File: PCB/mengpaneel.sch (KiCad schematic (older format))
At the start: 296 parts, among them IC1 MAX7219CNG+, IC10 STM32F411CEU7, IC11 AD5204BRUZ10-REEL7, IC12 LTC3631EMS8E#TRPBF, IC13 LMV321AUIDBVR, IC2 MAX7219CNG+, IC3 MTCH6301-I_ML, IC4 LTC3121EDE#PBF, IC5 AD5204BRUZ10-REEL7, IC6 AD5204BRUZ10-REEL7, IC7 LM3480IM3-3.3_NOPB, IC8 AD5204BRUZ10-REEL7, IC9 AD5204BRUZ10-REEL7, J1 UJ2-MIBH-G-SMT-TR, J2 Screw_Terminal_01x03, J3 Screw_Terminal_01x14, J4 SJ-63053A, J5 SJ-63053A, J6 SJ-63053A, J7 SJ-63053A, SW1 SW_Push, SW2 SW_DPDT_x2, SW3 SW_DPST_x2, SW4 SW_DPST_x2, U11 Touchpad_mp, U13 Touchpad_mp_LR, U14 Touchpad_mp, U15 Touchpad_mp, U16 Touchpad_mp, U17 Touchpad_mp, U2 Touchpad_mp, U3 Touchpad_mp, U4 Touchpad_mp, U5 LM324N, U6 Touchpad_mp, U7 LM324N, U8 Touchpad_mp, Y1 8MHz

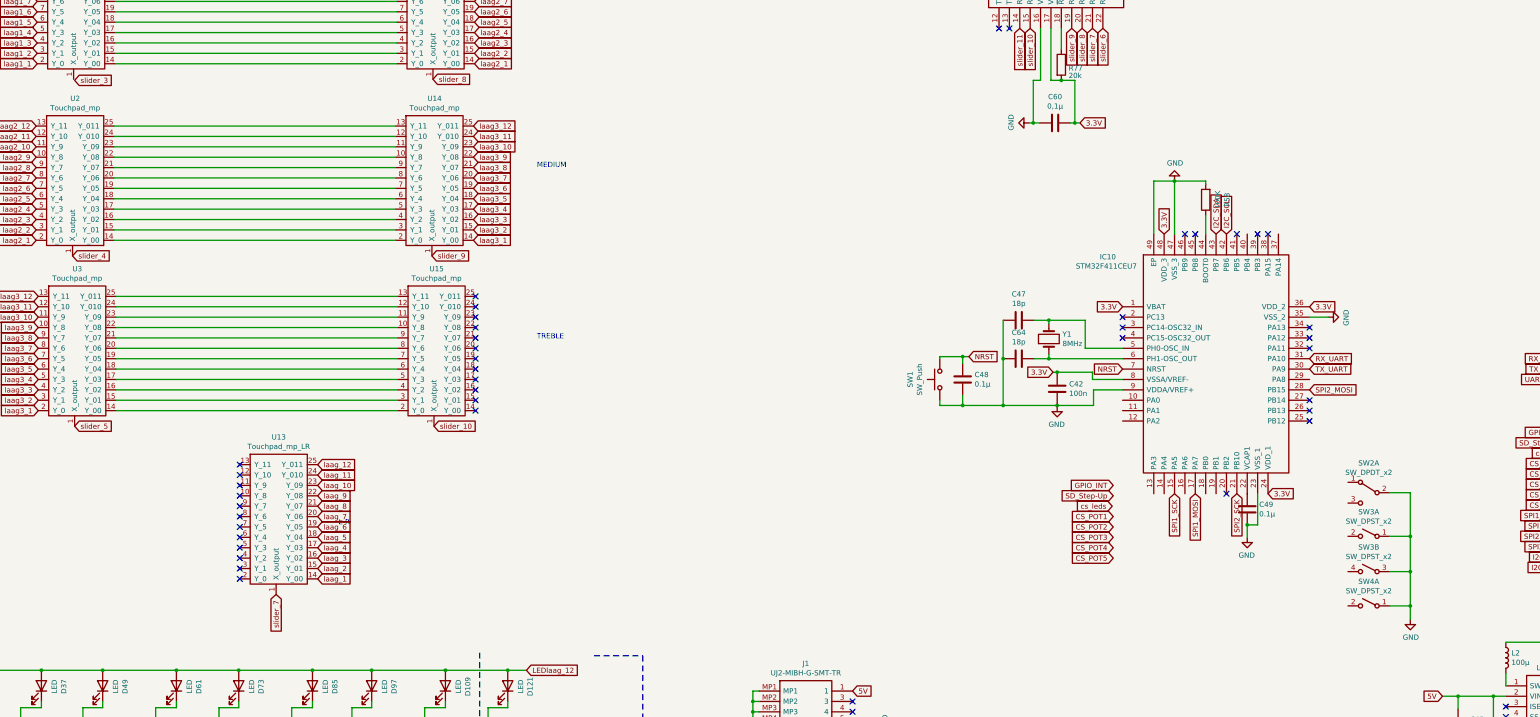
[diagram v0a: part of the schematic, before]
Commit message: PCB af nu wachten op de docenten hun feedback.
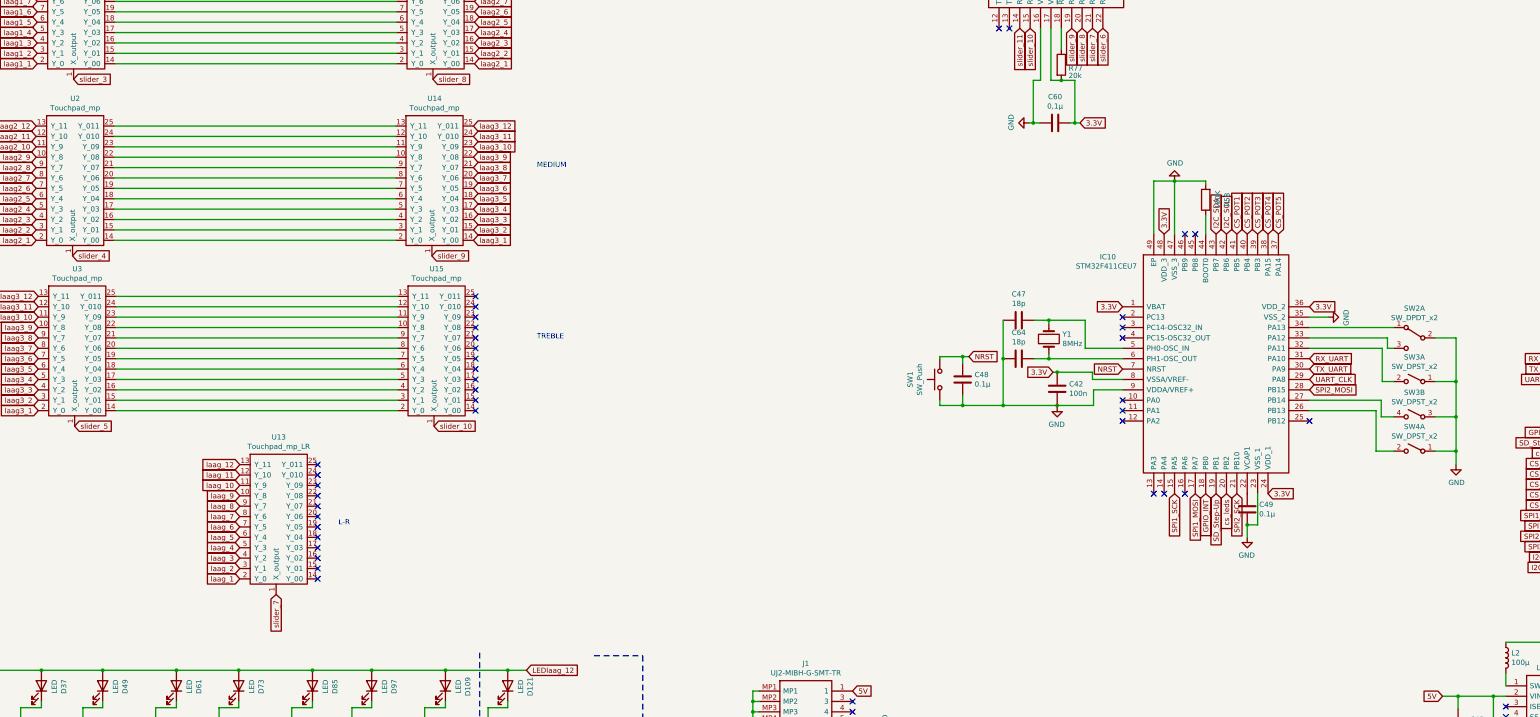
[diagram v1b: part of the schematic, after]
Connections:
- net CS_POT1: now also IC10.41 (PB5)
- net CS_POT2: now also IC10.40 (PB4)
- net CS_POT3: now also IC10.39 (PB3)
- net CS_POT4: now also IC10.38 (PA15)
- net CS_POT5: now also IC10.37 (PA14)
- net GPIO_INT: now also IC10.18 (PB0)
- net SD_Step-Up: now also IC10.19 (PB1)
- net UART_CLK: now also IC10.29 (PA8)
- net cs_leds: now also IC10.20 (PB2)
- net laag_1: now also U13.2 (Y_0); no longer U13.14 (Y_00)
- net laag_10: now also U13.11 (Y_9); no longer U13.23 (Y_09)
- net laag_11: now also U13.12 (Y_10); no longer U13.24 (Y_010)
- net laag_12: now also U13.13 (Y_11); no longer U13.25 (Y_011)
- net laag_2: now also U13.3 (Y_1); no longer U13.15 (Y_01)
- net laag_3: now also U13.4 (Y_2); no longer U13.16 (Y_02)
- net laag_4: now also U13.5 (Y_3); no longer U13.17 (Y_03)
- net laag_5: now also U13.6 (Y_4); no longer U13.18 (Y_04)
- net laag_6: now also U13.7 (Y_5); no longer U13.19 (Y_05)
- net laag_7: now also U13.8 (Y_6); no longer U13.20 (Y_06)
- net laag_8: now also U13.9 (Y_7); no longer U13.21 (Y_07)
- net laag_9: now also U13.10 (Y_8); no longer U13.22 (Y_08)
- net slider_3: now also U4.1 (X_output)
- net at SW2.1 (A): now also IC10.34 (PA13)
- net at SW2.3 (C): now also IC10.33 (PA12)
- net at SW3.2 (B): now also IC10.32 (PA11)
- net at IC10.26 (PB13): now also SW4.2 (B)
- net at IC10.27 (PB14): now also SW3.4 (B)
- no-connect marks 85 -> 82
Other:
- moved on the sheet: SW2A, SW3A, SW3B, SW4A
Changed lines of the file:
@@
 Text GLabel 19160 9880 0    50   Input ~ 0
 TX_UART
-Connection ~ 17650 12160
+Connection ~ 18090 10670
 Wire Wire Line
-	17650 12290 17650 12160
+	18090 10800 18090 10670
 Wire Wire Line
-	17650 11830 17650 12160
-Connection ~ 17650 11830
+	18090 10340 18090 10670
+Connection ~ 18090 10340
 Wire Wire Line
-	17650 11490 17650 11830
+	18090 10000 18090 10340
 Wire Wire Line
-	17650 12160 17450 12160
+	18090 10670 17890 10670
 $Comp
 L Switch:SW_DPST_x2 SW3
 U 2 1 8F2CC16C
-P 17250 11830
-F 0 "SW3" H 17250 12065 50  0000 C CNN
-F 1 "SW_DPST_x2" H 17250 11974 50  0000 C CNN
-F 2 "Connector_PinHeader_1.00mm:PinHeader_1x04_P1.00mm_Vertical" H 17250 11830 50  0001 C CNN
-F 3 "~" H 17250 11830 50  0001 C CNN
-	2    17250 11830
+P 17690 10340
+F 0 "SW3" H 17690 10575 50  0000 C CNN
+F 1 "SW_DPST_x2" H 17690 10484 50  0000 C CNN
+F 2 "Connector_PinHeader_1.00mm:PinHeader_1x04_P1.00mm_Vertical" H 17690 10340 50  0001 C CNN
+F 3 "~" H 17690 10340 50  0001 C CNN
+	2    17690 10340
 	-1   0    0    -1
 $EndComp
 Wire Wire Line
-	17650 11830 17450 11830
+	18090 10340 17890 10340
 $Comp
 L Switch:SW_DPST_x2 SW3
 U 1 1 603E27EC
-P 17250 11490
-F 0 "SW3" H 17250 11725 50  0000 C CNN
-F 1 "SW_DPST_x2" H 17250 11634 50  0000 C CNN
-F 2 "Connector_PinHeader_1.00mm:PinHeader_1x04_P1.00mm_Vertical" H 17250 11490 50  0001 C CNN
-F 3 "~" H 17250 11490 50  0001 C CNN
-	1    17250 11490
+P 17690 10000
+F 0 "SW3" H 17690 10235 50  0000 C CNN
+F 1 "SW_DPST_x2" H 17690 10144 50  0000 C CNN
+F 2 "Connector_PinHeader_1.00mm:PinHeader_1x04_P1.00mm_Vertical" H 17690 10000 50  0001 C CNN
+F 3 "~" H 17690 10000 50  0001 C CNN
+	1    17690 10000
 	-1   0    0    -1
 $EndComp
@@
 Text GLabel 4770 5400 2    50   Input ~ 0
 slider_2
-Text GLabel 4790 7100 2    50   Input ~ 0
+Text GLabel 4780 7090 2    50   Input ~ 0
 slider_3
 Text GLabel 8240 7090 2    50   Input ~ 0
@@
 NoConn ~ 13790 6600
 NoConn ~ 13690 6600
-Connection ~ 17650 11490
+Connection ~ 18090 10000
 $Comp
 L power:GND #PWR0198
 U 1 1 6059BB6E
-P 17650 12290
-F 0 "#PWR0198" H 17650 12040 50  0001 C CNN
-F 1 "GND" H 17655 12117 50  0000 C CNN
-F 2 "" H 17650 12290 50  0001 C CNN
-F 3 "" H 17650 12290 50  0001 C CNN
-	1    17650 12290
+P 18090 10800
+F 0 "#PWR0198" H 18090 10550 50  0001 C CNN
+F 1 "GND" H 18095 10627 50  0000 C CNN
+F 2 "" H 18090 10800 50  0001 C CNN
+F 3 "" H 18090 10800 50  0001 C CNN
+	1    18090 10800
 	1    0    0    -1
 $EndComp
 Wire Wire Line
-	17650 11490 17450 11490
+	18090 10000 17890 10000
 Wire Wire Line
-	17650 11070 17650 11490
+	18090 9580 18090 10000
 Wire Wire Line
-	17450 11070 17650 11070
+	17890 9580 18090 9580
 $Comp
 L Switch:SW_DPDT_x2 SW2
 U 1 1 603E0750
-P 17250 11070
-F 0 "SW2" H 17250 11355 50  0000 C CNN
-F 1 "SW_DPDT_x2" H 17250 11264 50  0000 C CNN
-F 2 "Connector_PinHeader_1.00mm:PinHeader_1x06_P1.00mm_Vertical" H 17250 11070 50  0001 C CNN
-F 3 "~" H 17250 11070 50  0001 C CNN
-	1    17250 11070
+P 17690 9580
+F 0 "SW2" H 17690 9865 50  0000 C CNN
+F 1 "SW_DPDT_x2" H 17690 9774 50  0000 C CNN
+F 2 "Connector_PinHeader_1.00mm:PinHeader_1x06_P1.00mm_Vertical" H 17690 9580 50  0001 C CNN
+F 3 "~" H 17690 9580 50  0001 C CNN
+	1    17690 9580
 	-1   0    0    -1
 $EndComp
@@
 	1    0    0    -1
 $EndComp
-$Comp
-L mengpaneel-rescue:STM32F411CEU7-STM32F411CEU7 IC10
-U 1 1 60AC800D
-P 14880 9280
-F 0 "IC10" H 14660 9760 50  0000 L CNN
-F 1 "STM32F411CEU7" H 14430 9700 50  0000 L TNN
-F 2 "STM32F411CEU7:QFN50P700X700X65-49N-D" H 16530 9780 50  0001 L CNN
-F 3 "https://componentsearchengine.com/Datasheets/2/STM32F411CEU7.pdf" H 16530 9680 50  0001 L CNN
-F 4 "STMICROELECTRONICS - STM32F411CEU7 - MCU, 32BIT, CORTEX-M4, 100MHZ, UFQFPN-48" H 16530 9580 50  0001 L CNN "Description"
-F 5 "0.65" H 16530 9480 50  0001 L CNN "Height"
-F 6 "511-STM32F411CEU7" H 16530 9380 50  0001 L CNN "Mouser Part Number"
-F 7 "https://www.mouser.co.uk/ProductDetail/STMicroelectronics/STM32F411CEU7/?qs=k5OWtXsTJaprF2FuhgNRlw%3D%3D" H 16530 9280 50  0001 L CNN "Mouser Price/Stock"
-F 8 "STMicroelectronics" H 16530 9180 50  0001 L CNN "Manufacturer_Name"
-F 9 "STM32F411CEU7" H 16530 9080 50  0001 L CNN "Manufacturer_Part_Number"
-	1    14880 9280
-	1    0    0    -1
-$EndComp
-NoConn ~ 15880 11080
-NoConn ~ 16680 10180
-NoConn ~ 16680 10280
 NoConn ~ 16680 10380
 NoConn ~ 15480 8580
 NoConn ~ 15580 8580
-NoConn ~ 15980 8580
-NoConn ~ 16180 8580
-NoConn ~ 16280 8580
-NoConn ~ 16680 9480
-NoConn ~ 16680 9580
-NoConn ~ 16680 9680
 NoConn ~ 14880 9480
 NoConn ~ 14880 9580
@@
 L Switch:SW_DPST_x2 SW4
 U 1 1 8F841806
-P 17250 12160
-F 0 "SW4" H 17250 12395 50  0000 C CNN
-F 1 "SW_DPST_x2" H 17250 12304 50  0000 C CNN
-F 2 "Connector_PinHeader_1.00mm:PinHeader_1x04_P1.00mm_Vertical" H 17250 12160 50  0001 C CNN
-F 3 "~" H 17250 12160 50  0001 C CNN
-	1    17250 12160
+P 17690 10670
+F 0 "SW4" H 17690 10905 50  0000 C CNN
+F 1 "SW_DPST_x2" H 17690 10814 50  0000 C CNN
+F 2 "Connector_PinHeader_1.00mm:PinHeader_1x04_P1.00mm_Vertical" H 17690 10670 50  0001 C CNN
+F 3 "~" H 17690 10670 50  0001 C CNN
+	1    17690 10670
 	-1   0    0    -1
 $EndComp
@@
 Text GLabel 19160 11690 0    50   Input ~ 0
 I2C_SCL
-Text GLabel 14790 11300 0    50   Input ~ 0
+Text GLabel 15980 8580 1    50   Input ~ 0
 CS_POT1
-Text GLabel 14780 11200 0    50   Input ~ 0
+Text GLabel 15880 11080 3    50   Input ~ 0
 cs_leds
-Text GLabel 14790 11000 0    50   Input ~ 0
+Text GLabel 15680 11080 3    50   Input ~ 0
 GPIO_INT
-Text GLabel 14790 11100 0    50   Input ~ 0
+Text GLabel 15780 11080 3    50   Input ~ 0
 SD_Step-Up
-Text GLabel 14790 11400 0    50   Input ~ 0
+Text GLabel 16080 8580 1    50   Input ~ 0
 CS_POT2
-Text GLabel 14790 11500 0    50   Input ~ 0
+Text GLabel 16180 8580 1    50   Input ~ 0
 CS_POT3
-Text GLabel 14790 11600 0    50   Input ~ 0
+Text GLabel 16280 8580 1    50   Input ~ 0
 CS_POT4
-Text GLabel 14790 11700 0    50   Input ~ 0
+Text GLabel 16380 8580 1    50   Input ~ 0
 CS_POT5
 Text GLabel 17970 20540 0    50   Input ~ 0
@@
 	1    0    0    -1
 $EndComp
-Text GLabel 7130 11900 2    50   Input ~ 0
+Text GLabel 6380 11900 0    50   Input ~ 0
 laag_1
-Text GLabel 7130 11800 2    50   Input ~ 0
+Text GLabel 6380 11800 0    50   Input ~ 0
 laag_2
-Text GLabel 7130 11700 2    50   Input ~ 0
+Text GLabel 6380 11700 0    50   Input ~ 0
 laag_3
-Text GLabel 7130 11600 2    50   Input ~ 0
+Text GLabel 6380 11600 0    50   Input ~ 0
 laag_4
-Text GLabel 7130 11500 2    50   Input ~ 0
+Text GLabel 6380 11500 0    50   Input ~ 0
 laag_5
-Text GLabel 7130 11400 2    50   Input ~ 0
+Text GLabel 6380 11400 0    50   Input ~ 0
 laag_6
-Text GLabel 7130 11300 2    50   Input ~ 0
+Text GLabel 6380 11300 0    50   Input ~ 0
 laag_7
-Text GLabel 7130 11200 2    50   Input ~ 0
+Text GLabel 6380 11200 0    50   Input ~ 0
 laag_8
-Text GLabel 7130 11100 2    50   Input ~ 0
+Text GLabel 6380 11100 0    50   Input ~ 0
 laag_9
-Text GLabel 7130 11000 2    50   Input ~ 0
+Text GLabel 6380 11000 0    50   Input ~ 0
 laag_10
-Text GLabel 7130 10900 2    50   Input ~ 0
+Text GLabel 6380 10900 0    50   Input ~ 0
 laag_11
-Text GLabel 7130 10800 2    50   Input ~ 0
+Text GLabel 6380 10800 0    50   Input ~ 0
 laag_12
 NoConn ~ 8650 9180
@@
 NoConn ~ 8650 10180
 NoConn ~ 8650 10280
-NoConn ~ 6380 10800
-NoConn ~ 6380 10900
-NoConn ~ 6380 11000
-NoConn ~ 6380 11100
-NoConn ~ 6380 11200
-NoConn ~ 6380 11300
-NoConn ~ 6380 11400
-NoConn ~ 6380 11500
-NoConn ~ 6380 11900
-NoConn ~ 6380 11800
-NoConn ~ 6380 11700
-NoConn ~ 6380 11600
+Text GLabel 16680 9980 2    50   Input ~ 0
+UART_CLK
+NoConn ~ 15480 11080
+NoConn ~ 15280 11080
+NoConn ~ 15180 11080
+NoConn ~ 14880 10180
+NoConn ~ 14880 10280
+NoConn ~ 14880 10380
+$Comp
+L mengpaneel-rescue:STM32F411CEU7-STM32F411CEU7 IC10
+U 1 1 60AC800D
+P 14880 9280
+F 0 "IC10" H 14660 9760 50  0000 L CNN
+F 1 "STM32F411CEU7" H 14430 9700 50  0000 L TNN
+F 2 "STM32F411CEU7:QFN50P700X700X65-49N-D" H 16530 9780 50  0001 L CNN
+F 3 "https://componentsearchengine.com/Datasheets/2/STM32F411CEU7.pdf" H 16530 9680 50  0001 L CNN
+F 4 "STMICROELECTRONICS - STM32F411CEU7 - MCU, 32BIT, CORTEX-M4, 100MHZ, UFQFPN-48" H 16530 9580 50  0001 L CNN "Description"
+F 5 "0.65" H 16530 9480 50  0001 L CNN "Height"
+F 6 "511-STM32F411CEU7" H 16530 9380 50  0001 L CNN "Mouser Part Number"
+F 7 "https://www.mouser.co.uk/ProductDetail/STMicroelectronics/STM32F411CEU7/?qs=k5OWtXsTJaprF2FuhgNRlw%3D%3D" H 16530 9280 50  0001 L CNN "Mouser Price/Stock"
+F 8 "STMicroelectronics" H 16530 9180 50  0001 L CNN "Manufacturer_Name"
+F 9 "STM32F411CEU7" H 16530 9080 50  0001 L CNN "Manufacturer_Part_Number"
+	1    14880 9280
+	1    0    0    -1
+$EndComp
+Wire Wire Line
+	16680 9480 17490 9480
+Wire Wire Line
+	17490 9680 17430 9680
+Wire Wire Line
+	17430 9680 17430 9580
+Wire Wire Line
+	17430 9580 16680 9580
+Wire Wire Line
+	16680 9680 17380 9680
+Wire Wire Line
+	17380 9680 17380 10000
+Wire Wire Line
+	17380 10000 17490 10000
+Wire Wire Line
+	16680 10180 17370 10180
+Wire Wire Line
+	17370 10180 17370 10340
+Wire Wire Line
+	17370 10340 17490 10340
+Wire Wire Line
+	16680 10280 17320 10280
+Wire Wire Line
+	17320 10280 17320 10670
+Wire Wire Line
+	17320 10670 17490 10670
+NoConn ~ 7130 11500
+NoConn ~ 7130 11600
+NoConn ~ 7130 11700
+NoConn ~ 7130 11800
+NoConn ~ 7130 11900
+NoConn ~ 7130 11400
+NoConn ~ 7130 11300
+NoConn ~ 7130 11200
+NoConn ~ 7130 11100
+NoConn ~ 7130 10800
+NoConn ~ 7130 10900
+NoConn ~ 7130 11000
 $EndSCHEMATC
